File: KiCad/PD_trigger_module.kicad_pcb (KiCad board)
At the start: 2 copper layers, 14 x 27.1 mm, 33 parts, among them J5 USB_C_Receptacle_USB2.0, Q1 AON7403, U1 HUSB238

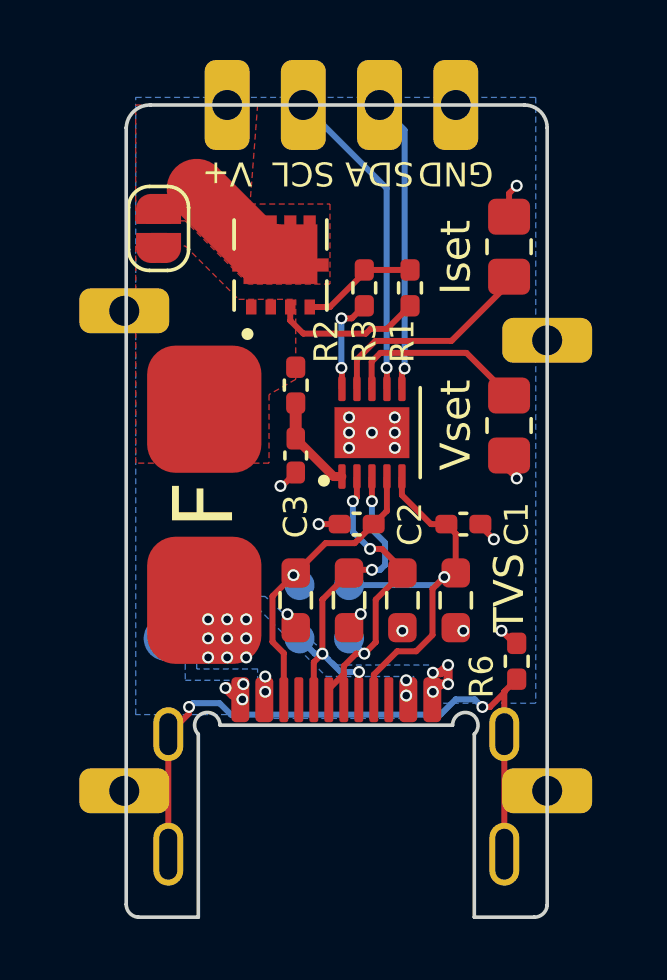
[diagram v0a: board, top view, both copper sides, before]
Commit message: Some minor corrections
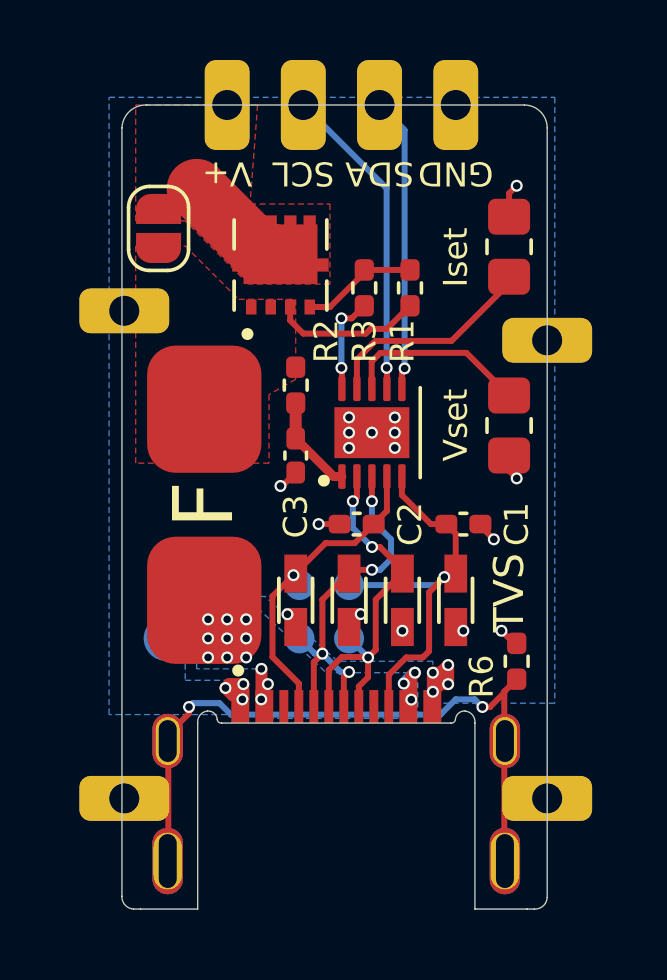
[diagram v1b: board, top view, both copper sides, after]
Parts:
- D1, D2, D3, D4: footprint Resistor_SMD:R_0603_1608Metric_Pad0.98x0.95mm_HandSolder -> _chips:ESD_PGB1010603MR
- J5: footprint _chips:USB_C_16pin -> _usb:TYPE_C_GCT_USB4505-03-0-A
- moved J5 4.23 mm to (147.7, 94.0)
- moved J2 0.25 mm to (154.7, 91.9)
- moved J2 0.25 mm to (140.6, 91.9)
- renumbered GND to J2
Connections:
- J2 pad 1: (no net) -> Vdd (x2)
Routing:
- net Net-(F1-Pad1): track 0.00 -> 2.48 mm, vias 13 -> 15
- net Net-(D1-Pad2): track 11.2 -> 12.8 mm
- net Vdd: track 8.07 -> 9.16 mm
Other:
- board size 14 x 27.1 mm -> 14.2 x 26.8 mm

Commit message: Design update
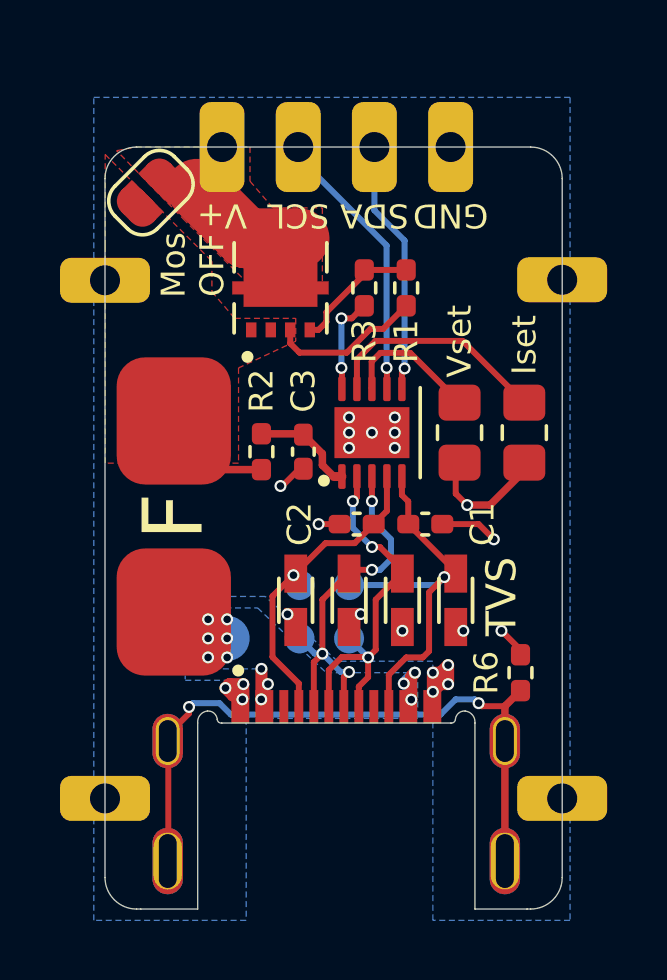
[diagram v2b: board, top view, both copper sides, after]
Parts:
- Ref**: moved to B.Cu
- moved Ref** 12.5 mm to (151.6, 89.9), turned to 90 degrees
- moved Iset 6.22 mm to (153.9, 79.8), turned to -90 degrees
- moved R2 2.50 mm to (145.2, 80.4), turned to 90 degrees
- moved J2 2.08 mm to (155.2, 74.7)
- moved Vset 1.67 mm to (151.8, 79.8)
- moved SDA 1.41 mm to (148.9, 70.2)
- moved GND 1.41 mm to (151.5, 70.2)
- moved SCL 1.41 mm to (146.4, 70.2)
- moved V+ 1.41 mm to (143.8, 70.2)
- moved C1 1.27 mm to (150.6, 82.8)
- moved JP1 1.22 mm to (141.5, 71.8), turned to 45 degrees
- moved J2 1.20 mm to (139.9, 74.7)
- moved F1 1.09 mm to (142.2, 82.5)
- moved Q1 0.76 mm to (145.8, 74.9)
- moved J2 0.64 mm to (139.9, 91.9)
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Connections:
- J2 pad 1: Net-(J5-PadS1) -> Vdd (x2)
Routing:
- net Vdd: track 9.16 -> 13.0 mm, vias 24 -> 23
- net Net-(F1-Pad2): track 5.01 -> 8.68 mm
- net Net-(R4-Pad1): track 6.20 -> 4.60 mm
- net SCL: track 10.6 -> 9.18 mm
- net SDA: track 9.80 -> 8.41 mm
- net Vss: track 3.43 -> 4.11 mm
- net Net-(F1-Pad1): vias 15 -> 12
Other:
- board size 14.2 x 26.8 mm -> 15.2 x 25.4 mm
- board text added: "Mos OFF"
